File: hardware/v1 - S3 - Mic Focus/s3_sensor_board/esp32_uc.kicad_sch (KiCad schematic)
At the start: 47 parts, among them J302 Micro_SD_Card_Det, J303 Conn_Coaxial, J304 UART, J305 EXT1, J306 EXT2, J307 I2C, J308 SPI, J309 USB_C_Receptacle_USB2.0_16P, SW301 BOOT, SW302 RST, U302 ESP32-C3, Y301 32kHz RTC Crystal, Y302 40 MHz

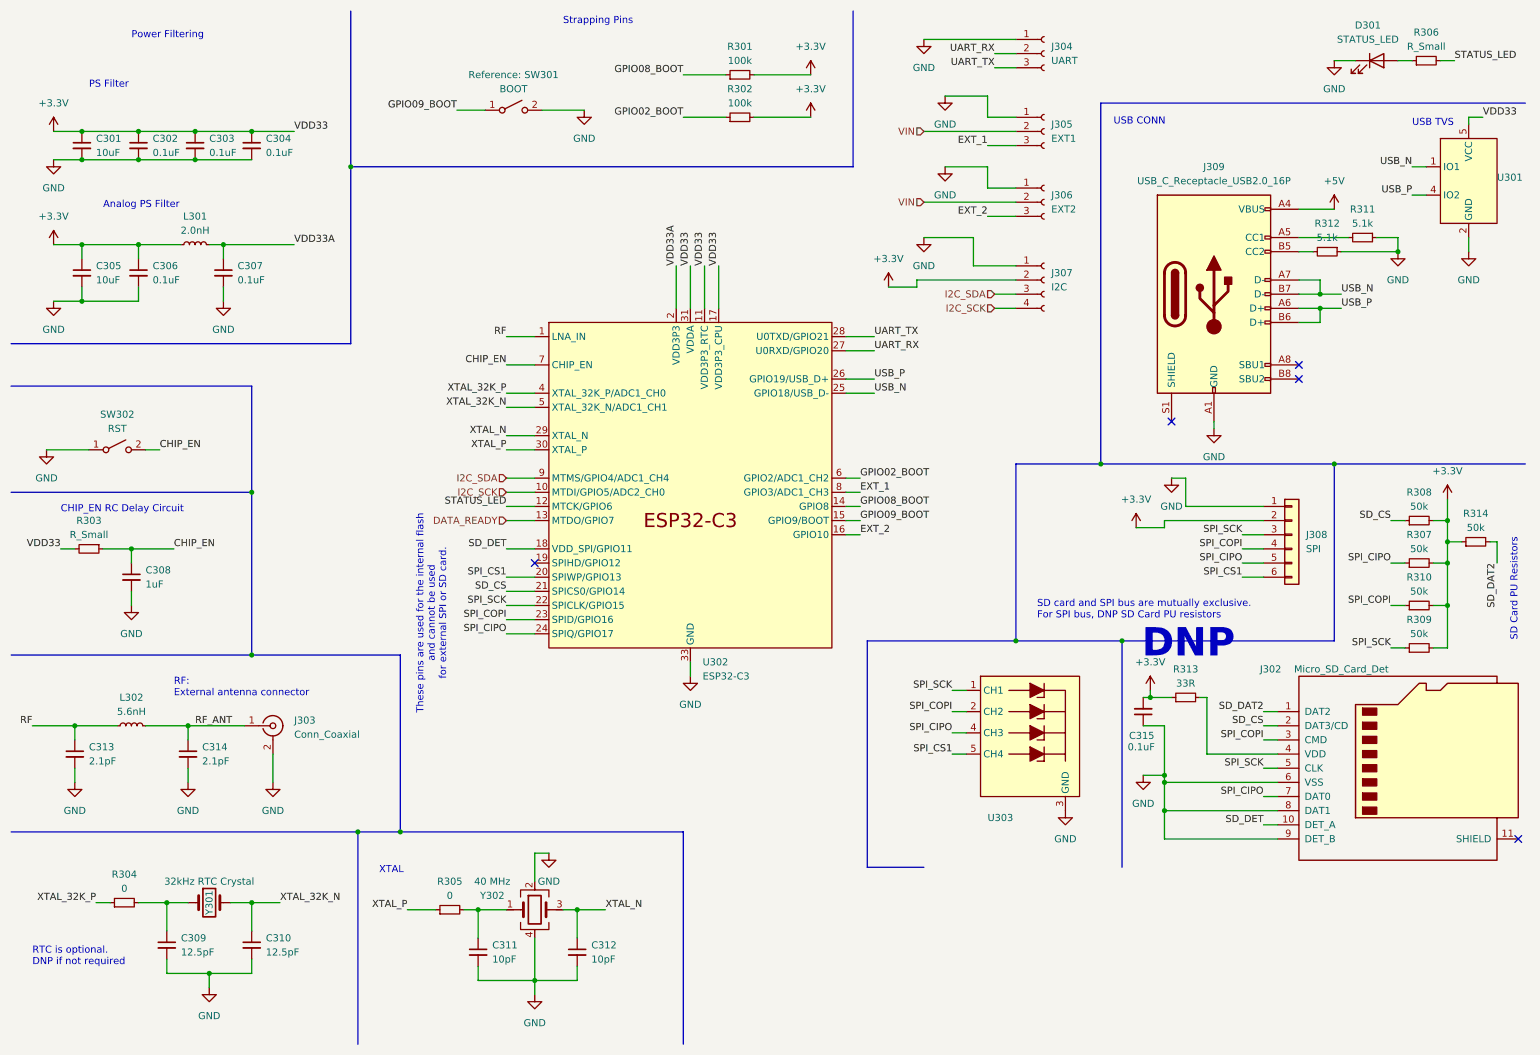
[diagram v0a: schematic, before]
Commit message: v1 board started
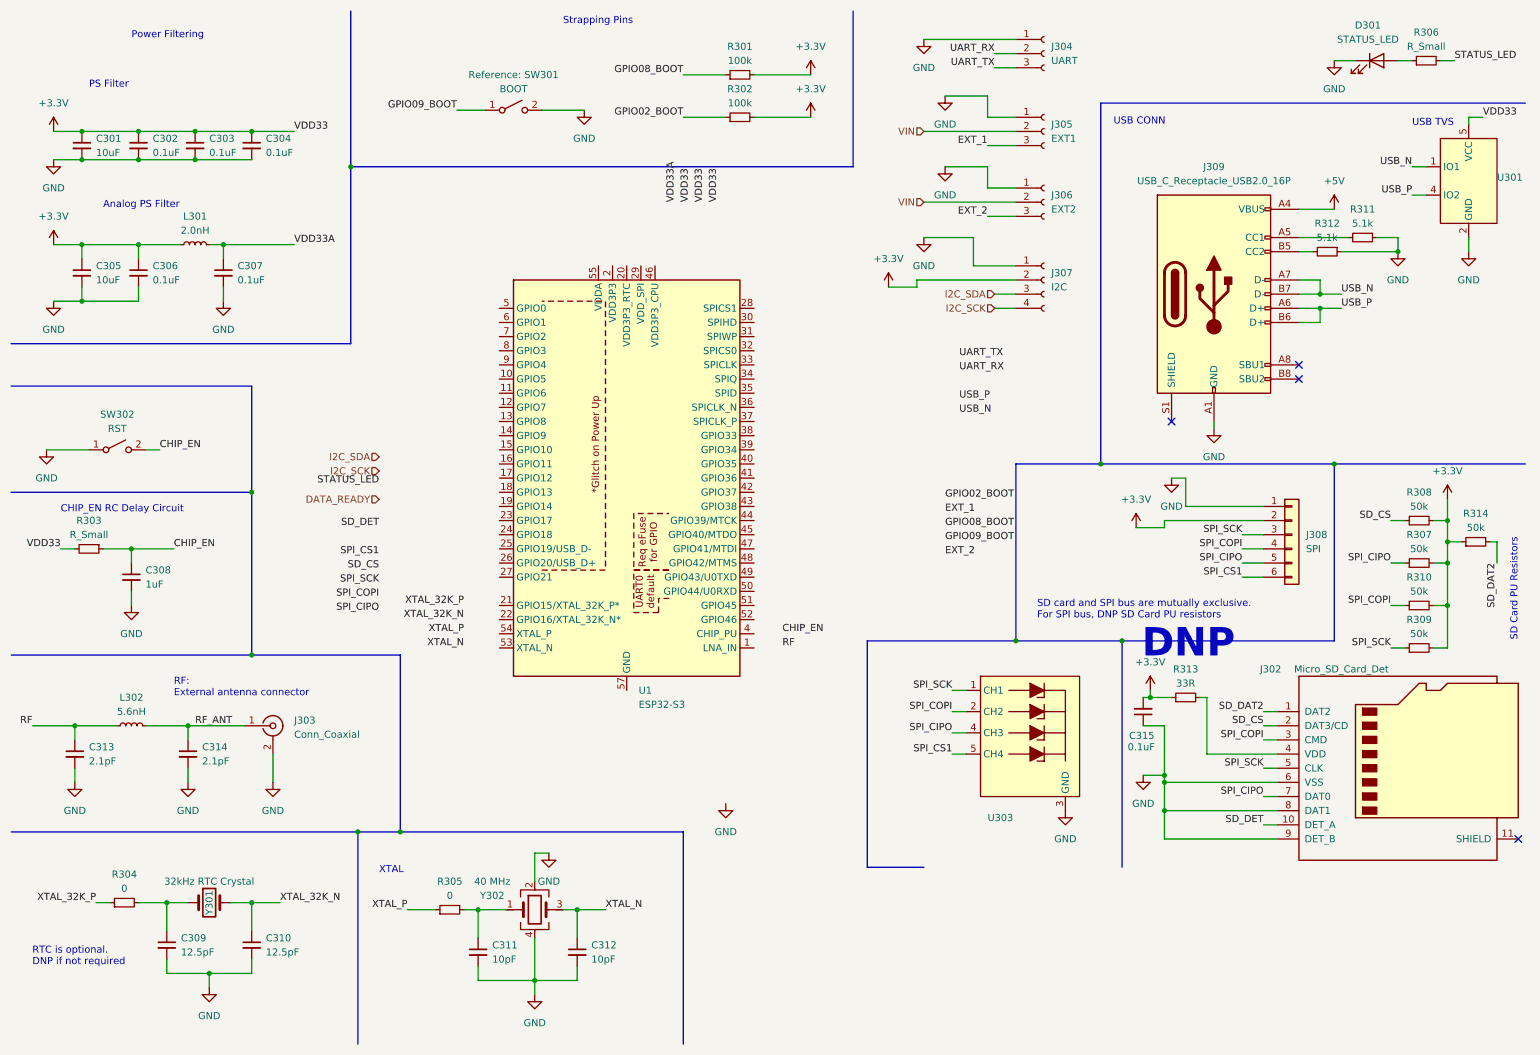
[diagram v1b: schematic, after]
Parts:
- removed U302: ESP32-C3, Package_DFN_QFN:QFN-32-1EP_5x5mm_P0.5mm_EP3.45x3.45mm, symbol Espressif:ESP32-C3
- added U1: ESP32-S3, Package_DFN_QFN:QFN-56-1EP_7x7mm_P0.4mm_EP4x4mm, symbol BVH Symbols:ESP32-S3
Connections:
- new net: U1.2 (VDD3P3), U1.3 (VDD3P3)
- new net: U1.55 (VDDA), U1.56 (VDDA)
- no-connect marks 5 -> 4
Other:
- note removed: "These pins are used for the internal flash and cannot be used for external SPI or SD card."
